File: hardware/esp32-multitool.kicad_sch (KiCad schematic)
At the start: 0 parts

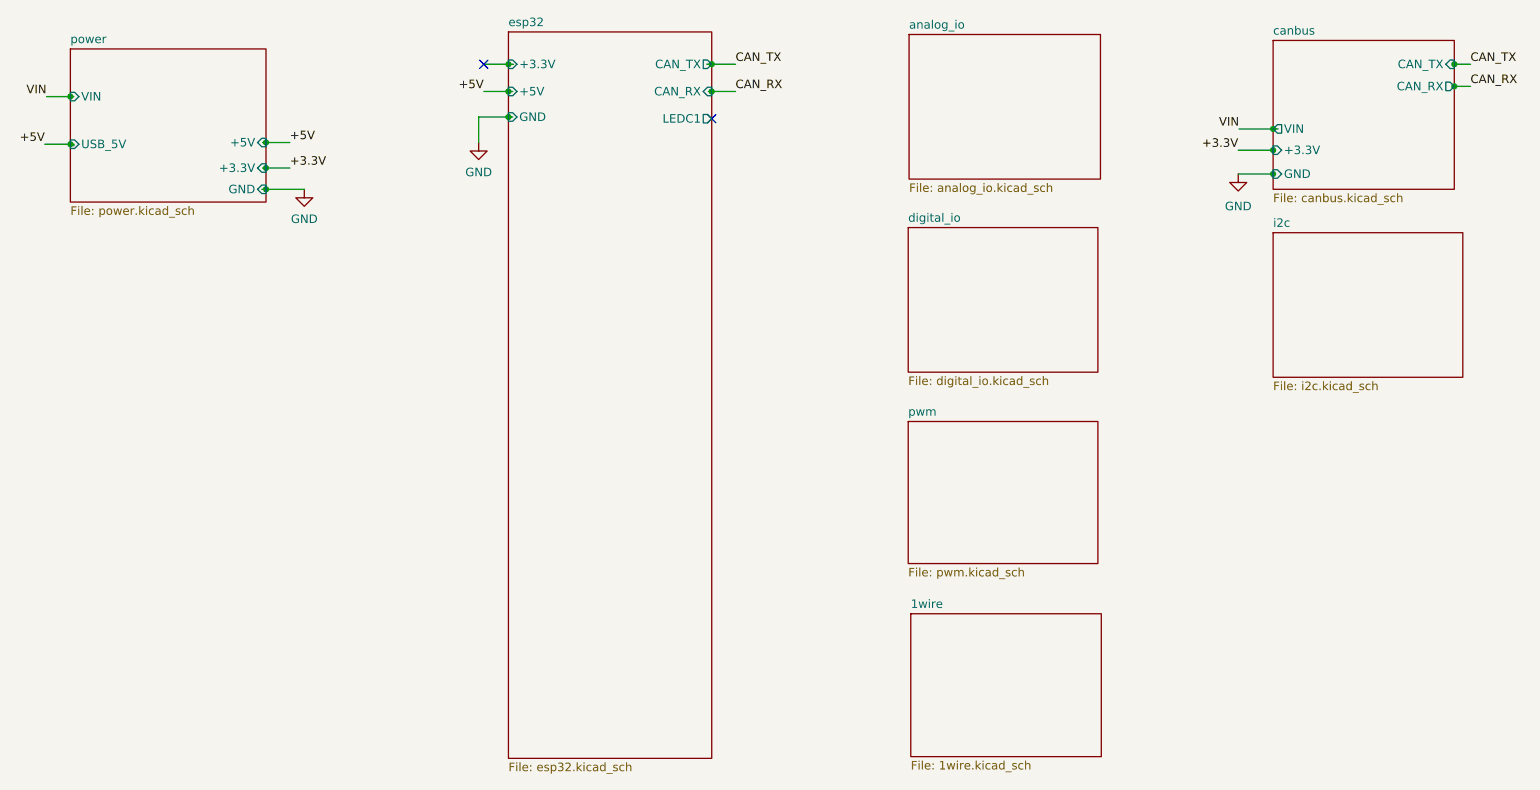
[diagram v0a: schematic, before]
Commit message: block refactoring
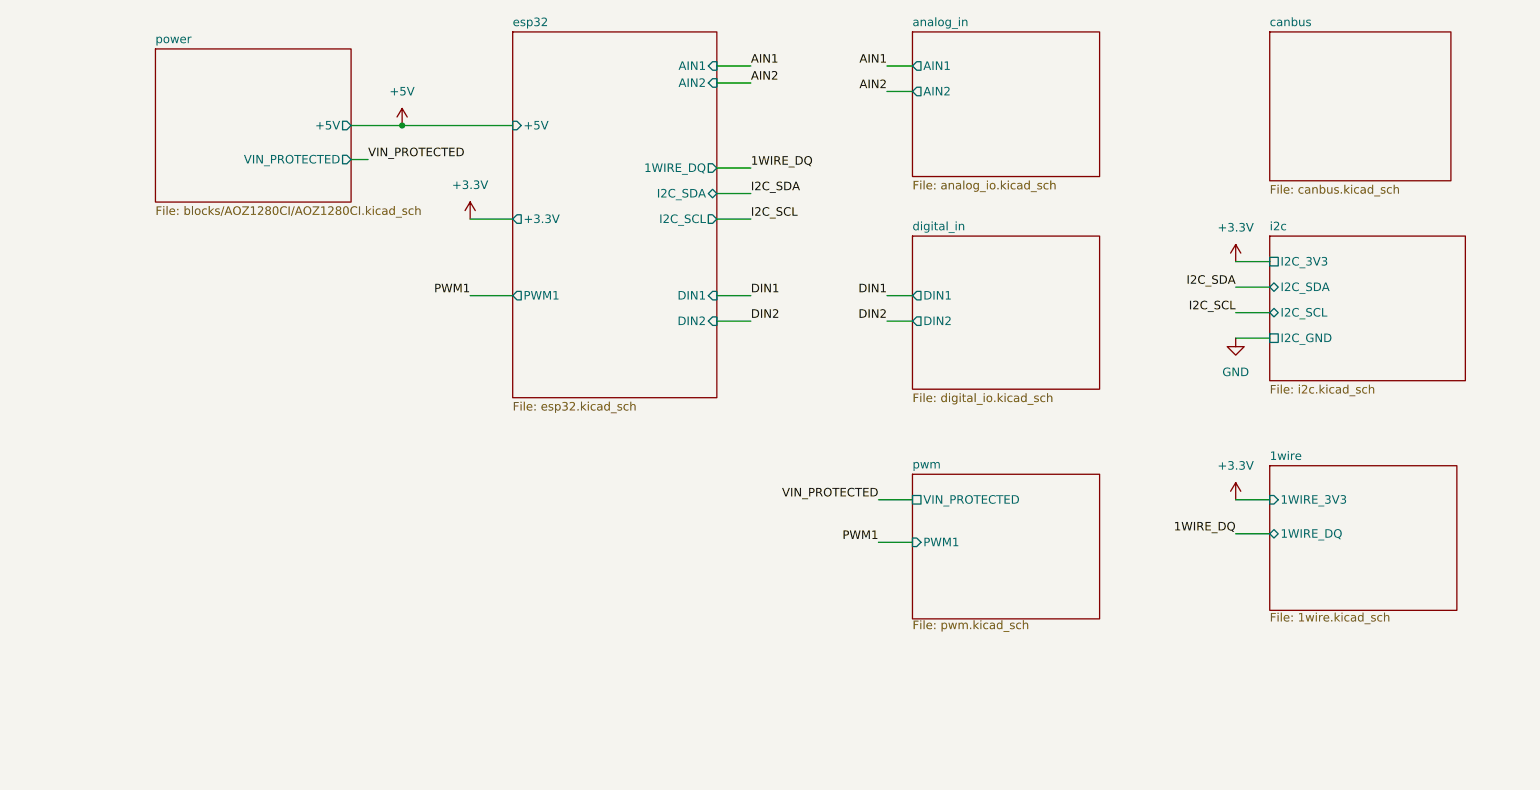
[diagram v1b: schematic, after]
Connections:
- no-connect marks 2 -> 0
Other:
- sheet analog_io renamed analog_in
- sheet digital_io renamed digital_in
- sheet 1wire ports: added 1WIRE_3V3, 1WIRE_DQ; removed none
- sheet analog_in ports: added AIN1, AIN2; removed none
- sheet canbus ports: added none; removed +3.3V, CAN_RX, CAN_TX, GND, VIN
- sheet digital_in ports: added DIN1, DIN2; removed none
- sheet esp32 ports: added 1WIRE_DQ, AIN1, AIN2, DIN1, DIN2, I2C_SCL, I2C_SDA, PWM1; removed CAN_RX, CAN_TX, GND, LEDC1
- sheet i2c ports: added I2C_3V3, I2C_GND, I2C_SCL, I2C_SDA; removed none
- sheet power: file power.kicad_sch -> blocks/AOZ1280CI/AOZ1280CI.kicad_sch
- sheet power ports: added VIN_PROTECTED; removed +3.3V, GND, USB_5V, VIN
- sheet pwm ports: added PWM1, VIN_PROTECTED; removed none
